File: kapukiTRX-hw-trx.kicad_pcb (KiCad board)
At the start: 4 copper layers, 45.7 x 27.9 mm, 87 parts, among them J1 GPS, J10 Conn_01x01, J11 Conn_01x01, J12 Conn_01x01, J13 Conn_01x01, J14 Conn_01x01, J15 Conn_01x01, J16 Conn_01x01, J17 Conn_01x01, J18 Conn_01x01, J19 GND for the Servo connectors, J2 SWD, J20 CAN, J3 Conn_01x01, J4 Conn_01x01, J5 Conn_01x01, J6 Conn_01x01, J7 Conn_01x01, J8 Conn_01x01, J9 Conn_01x01, U1 STM32G474VE, U2 LP38693-3.3, U3 TXB0108PWR, U4 LP38693-5.0, U5 MCP2562-E-MF, U6 LP38693SD-3.3, U7 BNO055, Y1 16MHz, Y2 32.768kHz

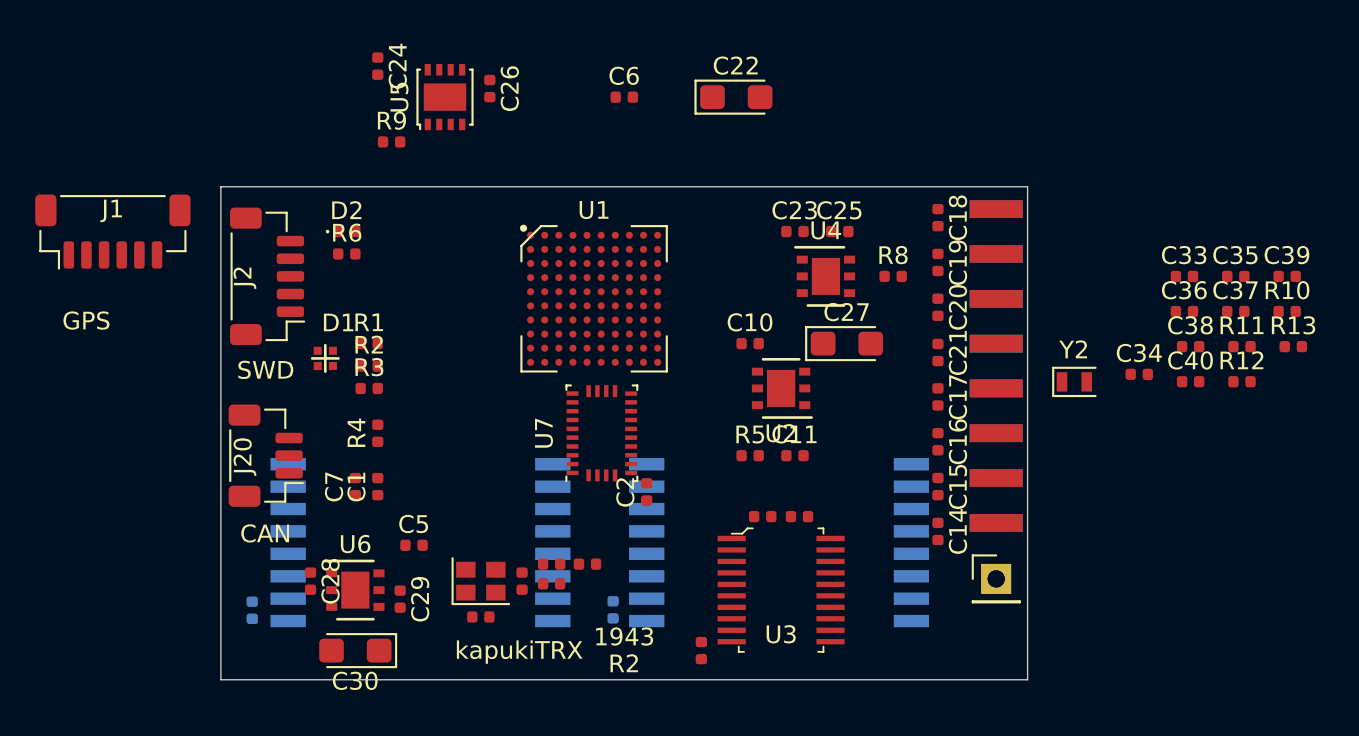
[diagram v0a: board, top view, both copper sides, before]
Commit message: Placing components and start routing
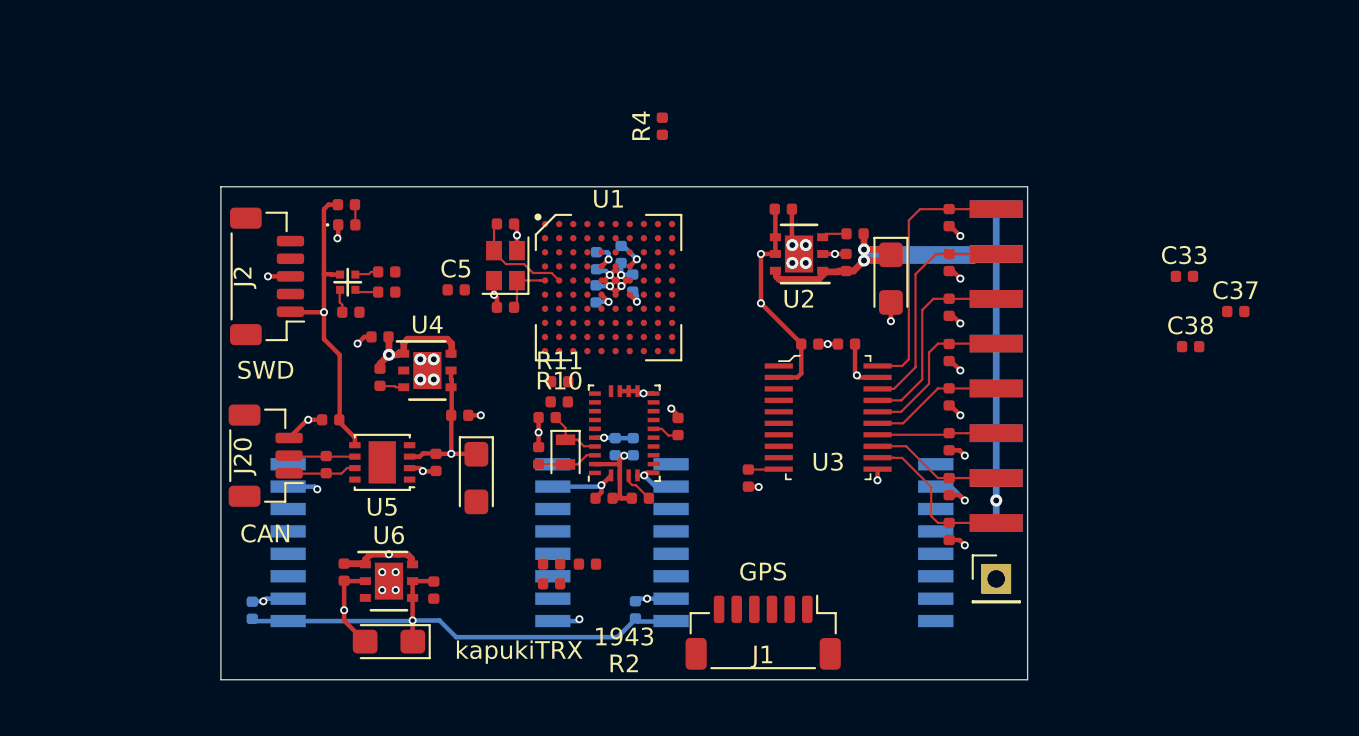
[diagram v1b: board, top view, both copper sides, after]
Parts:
- C1, C2, C35, C36, C6, C7, J10, J12, J14, J16, J18, J4, J6, J8: moved to B.Cu
- J11, J13, J15, J17, J3, J5, J7, J9: moved to F.Cu
- moved J1 43.3 mm to (202.2, 119.3), turned to 180 degrees
- moved C39 42.7 mm to (189.9, 107.1)
- moved R10 41.6 mm to (190.6, 106.2)
- moved R11 38.7 mm to (190.7, 105.0)
- moved C40 37.2 mm to (189.5, 109.2), turned to 270 degrees
- moved C35 36.5 mm to (193.8, 108.7), turned to 270 degrees
- moved R13 35.2 mm to (197.4, 107.6), turned to 270 degrees
- moved R12 34.7 mm to (195.2, 111.6)
- moved C36 32.2 mm to (194.8, 108.7), turned to 270 degrees
- moved C34 31.1 mm to (193.2, 111.6), turned to 180 degrees
- moved R8 29.6 mm to (180.5, 104.8), turned to 90 degrees
- moved Y2 29.1 mm to (191.0, 109.0), turned to 270 degrees
- moved C23 24.3 mm to (180.5, 102.5), turned to 180 degrees
- moved C25 23.9 mm to (185.0, 106.9)
- moved R4 23.7 mm to (196.5, 90.6)
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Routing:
- net IN: track 0.00 -> 106.8 mm, vias 0 -> 5
- net /VCCCPU: track 0.00 -> 88.3 mm, vias 0 -> 9
- net GND: track 0.00 -> 62.4 mm, vias 0 -> 47
- net /Connectors/VCCOUT: track 0.00 -> 37.0 mm, vias 0 -> 2
- net /RF modules/VCCRF: track 0.00 -> 29.4 mm, vias 0 -> 1
- net Net-(C18-Pad1): track 0.00 -> 15.0 mm
- net Net-(C19-Pad1): track 0.00 -> 13.0 mm
- net Net-(C20-Pad1): track 0.00 -> 11.4 mm
- net Net-(C21-Pad1): track 0.00 -> 9.37 mm
- net Net-(C14-Pad1): track 0.00 -> 9.22 mm
- net Net-(C17-Pad1): track 0.00 -> 7.54 mm
- net Net-(C15-Pad1): track 0.00 -> 7.47 mm
- net Net-(C16-Pad1): track 0.00 -> 6.76 mm
- net Net-(C4-Pad1): track 0.00 -> 6.07 mm
- net Net-(J20-Pad1): track 0.00 -> 3.91 mm
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- added copper zone on In1.Cu, net GND
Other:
- net class Default: via_dia 0.508 -> 0.4572
- net class IN added: clearance 0.2032, trace_width 0.381, via_dia 0.6858, via_drill 0.3302
- net class VCC added: clearance 0.1524, trace_width 0.254, via_dia 0.4572, via_drill 0.254
- rule pad_to_mask_clearance: 0.051 -> 0.0508
- rule solder_mask_min_width: 0.25 -> 0.1016
- rule via_min_size: 0.508 -> 0.4572
